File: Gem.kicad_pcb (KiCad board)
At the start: 2 copper layers, 76.2 x 54.6 mm, 39 parts, among them IC1 AD8226, IC2 AD8538ARZ, M1 ALLSENSORS-A6AAF-CUTLEADS, M2 DIAVOLINO, M3 POLOLU-MICROSD, M4 POLOLU-REGULATOR-MOD, M5 ADAFRUIT-ADS1115-MOD, M6 ADAFRUIT-GPS-MOD

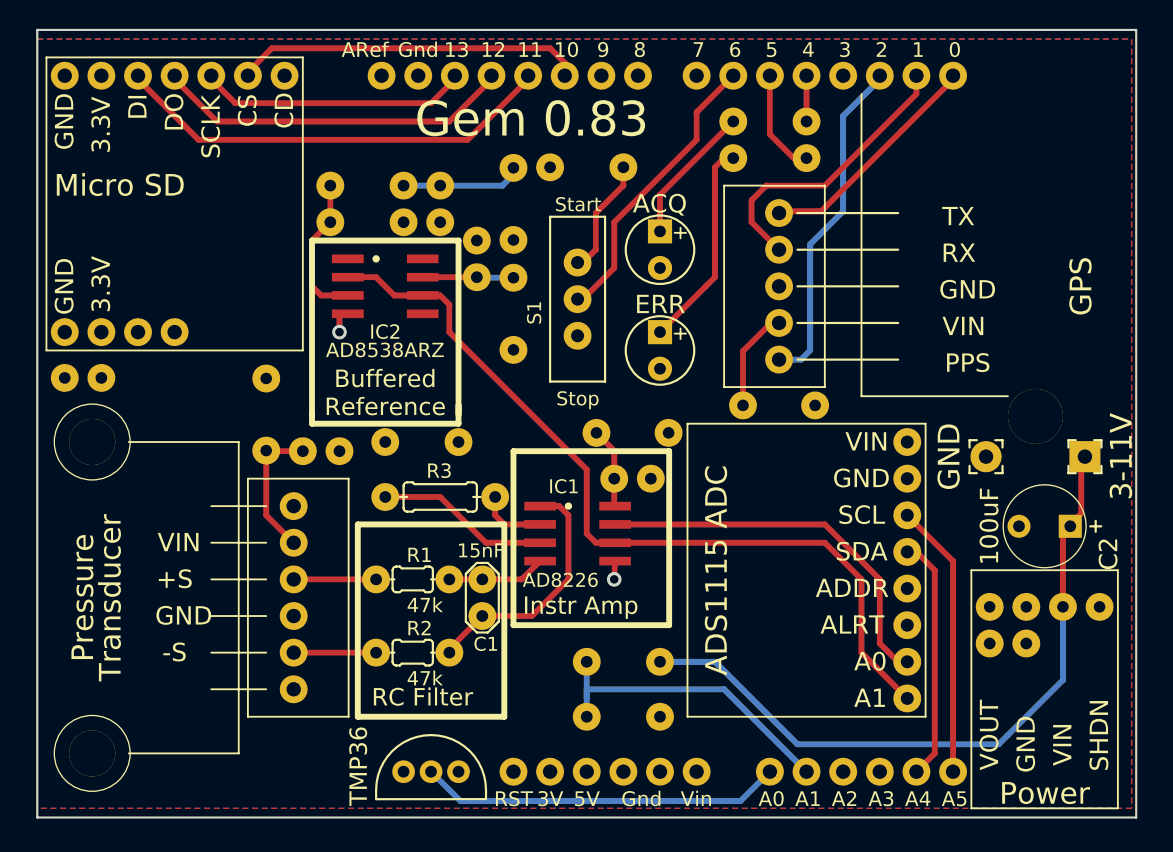
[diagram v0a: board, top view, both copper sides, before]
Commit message: v0.9, first version using Efficientino
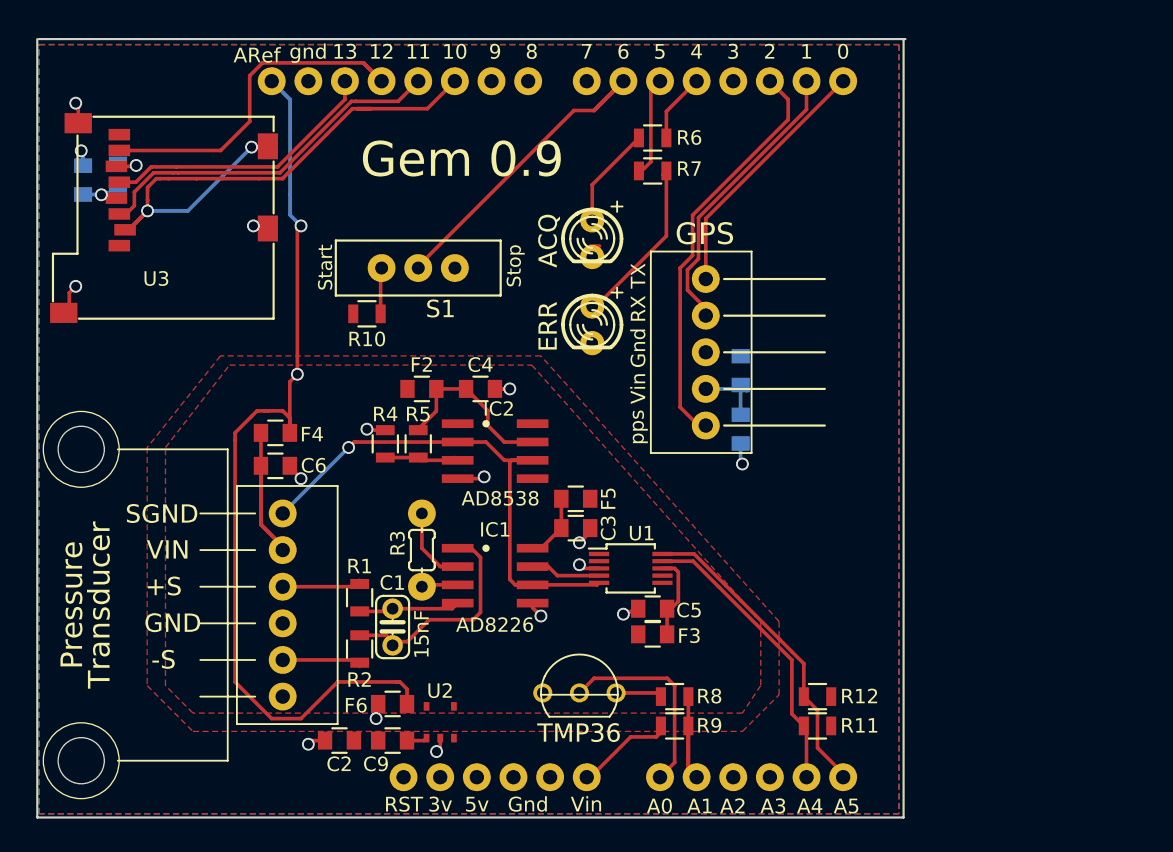
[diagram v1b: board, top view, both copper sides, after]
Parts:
- removed 2-11V37, GND37: WIREPAD2,15/1,0, 2_15_1_0
- removed C7: 0.1uF, C025-024X044
- removed M3: POLOLU-MICROSD, POLOLU-MICROSD
- removed M4: POLOLU-REGULATOR-MOD, POLOLU-ADJUSTABLE-REGULATOR-MOD
- removed M5: ADAFRUIT-ADS1115-MOD, ADAFRUIT-ADS1115-MOD
- removed hole: VAL**, hole
- added C10: 0.1uF, Capacitors_SMD:C_0805, B.Cu at (48.8, 23.0)
- added F6: FB, Capacitors_SMD:C_0805, F.Cu at (24.6, 48.6)
- added F7: FB, Capacitors_SMD:C_0805, B.Cu at (3.17, 9.78)
- added R11: 2.2k, Resistors_SMD:R_0805, F.Cu at (54.1, 45.6)
- added R12: 2.2k, Resistors_SMD:R_0805, F.Cu at (54.1, 47.6)
- added U1: ADS1115, Housings_SSOP:MSOP-10_3x3mm_Pitch0.5mm, F.Cu at (41.1, 36.7)
- added U2: TCR2EF, Gem-modular:SC-74A, F.Cu at (27.9, 47.4)
- added U3: Micro-SD, Gem-modular:Micro-SD, F.Cu at (0.89, 19.7)
- C1: footprint C025-024X044 -> Gem-modular:C025-024X044
- C2: value 100uF -> 0.1uF; footprint E3_5-8 -> Capacitors_SMD:C_0805
- C3, C4, C5, C6: footprint C025-024X044 -> Capacitors_SMD:C_0805; moved to F.Cu
- C8: footprint C025-024X044 -> Capacitors_SMD:C_0805
- C9: value 22uF -> 22 uF; footprint C050-024X044 -> Capacitors_SMD:C_0805; moved to F.Cu
- F1: footprint FB -> Capacitors_SMD:C_0805
- F2, F3, F4, F5: footprint FB -> Capacitors_SMD:C_0805; moved to F.Cu
- IC1: footprint SO8 -> Gem-modular:SO8
- IC2: value AD8538ARZ -> AD8538; footprint SO8 -> Gem-modular:SO8
- M1: footprint ALLSENSORS-A6AAF-CUTLEADS -> Gem-modular:ALLSENSORS-A6AAF-CUTLEADS
- M2: footprint ARDUINO-NOHOLE-DIM_ON_BDOCU_ONLY_movetext -> Gem-modular:ARDUINO-NOHOLE-DIM_ON_BDOCU_ONLY
- M6: footprint ADAFRUIT-ULTIMATE-GPS-MOD -> Gem-modular:ADAFRUIT-ULTIMATE-GPS-MOD
- R1, R2: footprint 0204_5 -> Resistors_SMD:R_0805
- R10, R4, R5, R6, R7, R8, R9: footprint 0204_5 -> Resistors_SMD:R_0805; moved to F.Cu
- R3: footprint 0204_7 -> Gem-modular:0204_5
- S1: footprint EG1218 -> Gem-modular:EG1218
- TMP36: footprint TO92-EBC-OVAL -> Gem-modular:TO92-EBC-OVAL
- red1: footprint LED3MM -> Gem-modular:LED3MM
- moved C2 51.1 mm to (21.0, 48.6)
- moved C5 31.7 mm to (42.7, 39.5), turned to 0 degrees
- moved F3 31.4 mm to (42.7, 41.3), turned to 0 degrees
- moved R10 18.3 mm to (22.9, 19.1)
- moved C9 18.3 mm to (24.6, 46.1)
- moved R4 18.3 mm to (26.4, 28.1), turned to 90 degrees
- moved R5 15.4 mm to (24.1, 28.1), turned to 270 degrees
- moved C8 14.1 mm to (5.59, 9.65), turned to 270 degrees
- moved IC2 13.7 mm to (31.8, 28.6)
- moved TMP36 12.5 mm to (37.6, 44.1), turned to 0 degrees
- moved S1 11.3 mm to (26.4, 15.9), turned to 0 degrees
- moved C4 9.02 mm to (30.7, 24.3), turned to 0 degrees
- moved F2 8.21 mm to (26.7, 24.3), turned to 0 degrees
- moved R7 8.21 mm to (42.7, 6.86)
- moved R6 8.18 mm to (42.7, 9.14), turned to 0 degrees
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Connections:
- C4 pad 1: /N$30 -> /N$29
- C5 pad 1: /N$29 -> GND
- C5 pad 2: GND -> Net-(C5-Pad2)
- C8 pad 1: +3V3 -> GND
- C8 pad 2: GND -> Net-(C8-Pad2)
- C9 pad 1: +3V3 -> VAA
- IC1 pad 6: /N$10 -> +1V5
- IC2 pad 2: /N$10 -> +1V5
- IC2 pad 6: /N$10 -> +1V5
- IC2 pad 7: /N$30 -> /N$29
- M1 pad 1: (no net) -> +1V5
- M2 pad 5V: +3V3 -> Net-(M2-Pad5V)
- M2 pad A2: (no net) -> Net-(M2-PadA2)
- M2 pad A3: (no net) -> Net-(M2-PadA3)
- M2 pad AREF: (no net) -> VAA
- M2 pad D3: (no net) -> Net-(M2-PadD3)
- M2 pad D7: (no net) -> Net-(M2-PadD7)
- M2 pad D8: (no net) -> Net-(M2-PadD8)
- M2 pad D9: (no net) -> Net-(M2-PadD9)
- M2 pad RESE: (no net) -> Net-(M2-PadRESE)
- M2 pad VIN: (no net) -> +BATT
- R8 pad 1: /N$1 -> +BATT
- TMP36 pad E: +3V3 -> VAA
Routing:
- net VAA: track 0.00 -> 63.9 mm, vias 0 -> 2
- net /N$10: track 57.6 -> 0.00 mm
- net /N$1: track 48.5 -> 0.00 mm
- net +1V5: track 0.00 -> 36.1 mm, vias 0 -> 1
- net /N$2: track 26.8 -> 4.86 mm
- net GND: track 3.24 -> 25.1 mm, vias 2 -> 15
- net /N$11: track 24.3 -> 41.4 mm, vias 0 -> 2
- net /N$27: track 22.1 -> 9.11 mm
- net /N$25: track 25.2 -> 14.0 mm
- net /N$5: track 12.1 -> 2.53 mm
- net +BATT: track 0.00 -> 6.88 mm
- net /N$30: track 6.31 -> 0.00 mm
- net Net-(C5-Pad2): track 0.00 -> 6.01 mm
- net /N$12: track 31.1 -> 25.2 mm
- net /N$18: track 23.5 -> 28.8 mm
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- added copper zone on F.Cu, net VAA
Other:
- board size 76.2 x 54.6 mm -> 60.2 x 54 mm
- net class Default: clearance 0.3048 -> 0.1524; trace_width 0.4064 -> 0.254
- rule trace_clearance: 0.3048 -> 0.1524
- rule trace_min: 0.4064 -> 0.1524
- board text added: "Gem 0.9"
- board text removed: "Buffered Reference"
- board text removed: "Gem 0.83"
- board text removed: "Instr Amp"
- board text removed: "RC Filter"
